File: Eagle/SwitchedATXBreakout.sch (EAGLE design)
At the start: 51 parts, among them K1 ALF1P05, K2 ALF1P05, K3 ALF1P05, K4 ALF1P05, K5 ALF1P05, X1 22-23-2091, X2 5566-24

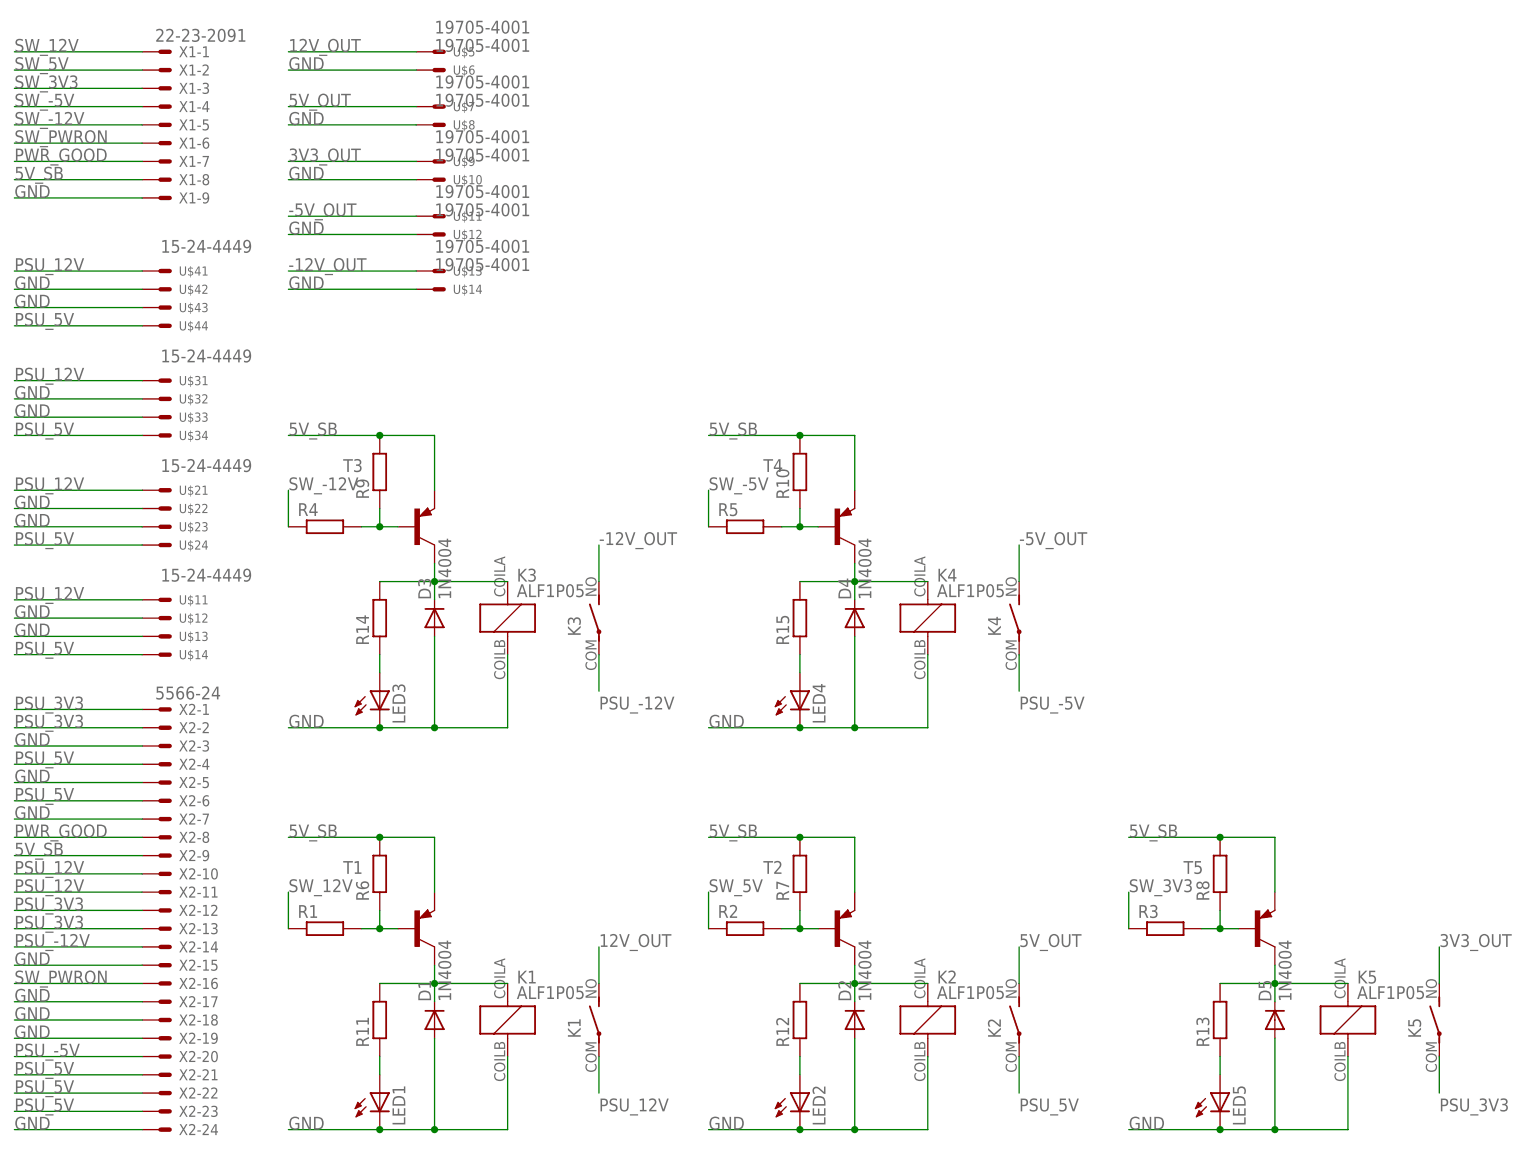
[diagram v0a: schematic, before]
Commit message: Start board layout
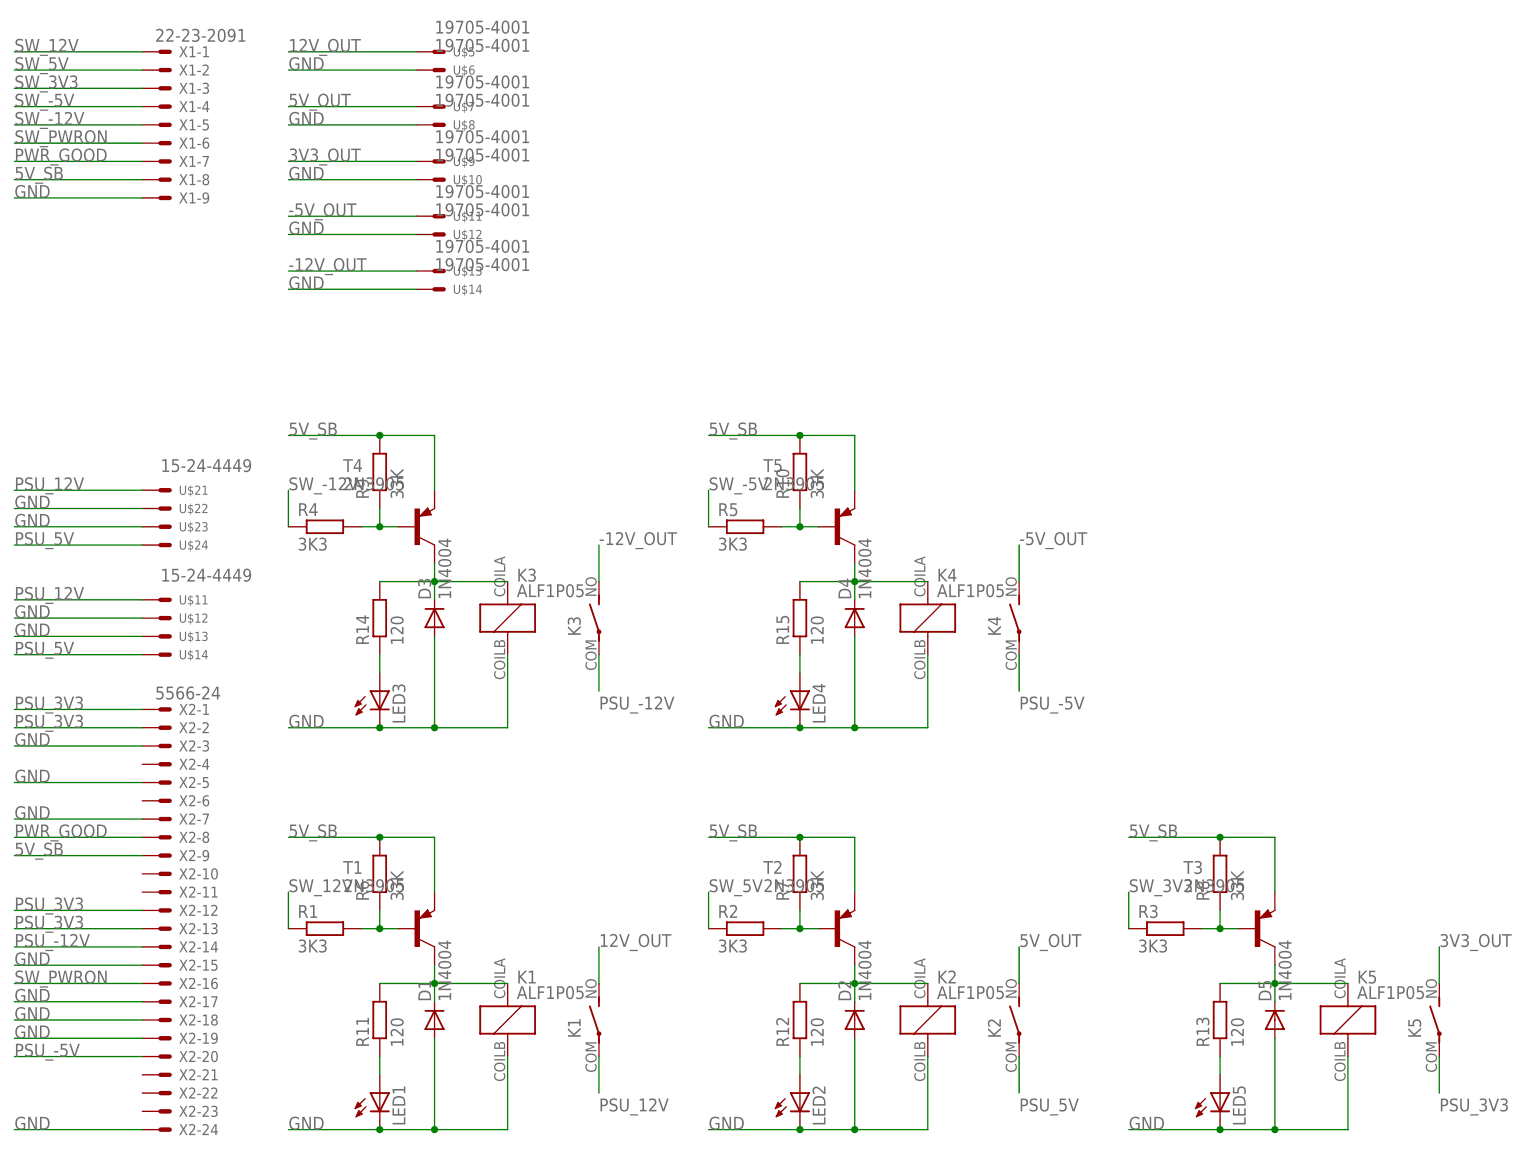
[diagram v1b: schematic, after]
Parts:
- removed U$3, U$4: 15-24-4449, con-molex-additional:15-24-4449
- LED1, LED2, LED3, LED4, LED5: device led:LED5MM -> led:LED3MM
- R1, R2, R3, R4, R5: value (none) -> 3K3; device resistor:R-EU_0204/5 -> resistor:R-EU_0204/7
- R10, R6, R7, R8, R9: value (none) -> 33K; device resistor:R-EU_0204/5 -> resistor:R-EU_0204/7
- R11, R12, R13, R14, R15: value (none) -> 120; device resistor:R-EU_0204/5 -> resistor:R-EU_0204/7
- T1, T2, T3, T4, T5: value (none) -> 2N3905; device transistor:-PNP-TO92 -> transistor:BC636-PNP-TO92-BCE
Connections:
- net GND: no longer U$32.P$1, U$33.P$1, U$42.P$1, U$43.P$1
- net N$11: now also T5.C; no longer T4.C
- net N$14: now also T3.C; no longer T5.C
- net N$2: now also T4.B; no longer T3.B
- net N$5: now also T5.B; no longer T4.B
- net N$7: now also T3.B; no longer T5.B
- net N$8: now also T4.C; no longer T3.C
- net PSU_12V: no longer U$31.P$1, U$41.P$1, X2-10.S, X2-11.S
- net PSU_5V: no longer U$34.P$1, U$44.P$1, X2-21.S, X2-22.S, X2-23.S, X2-4.S, X2-6.S
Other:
- moved on the sheet: T3, T4, T5

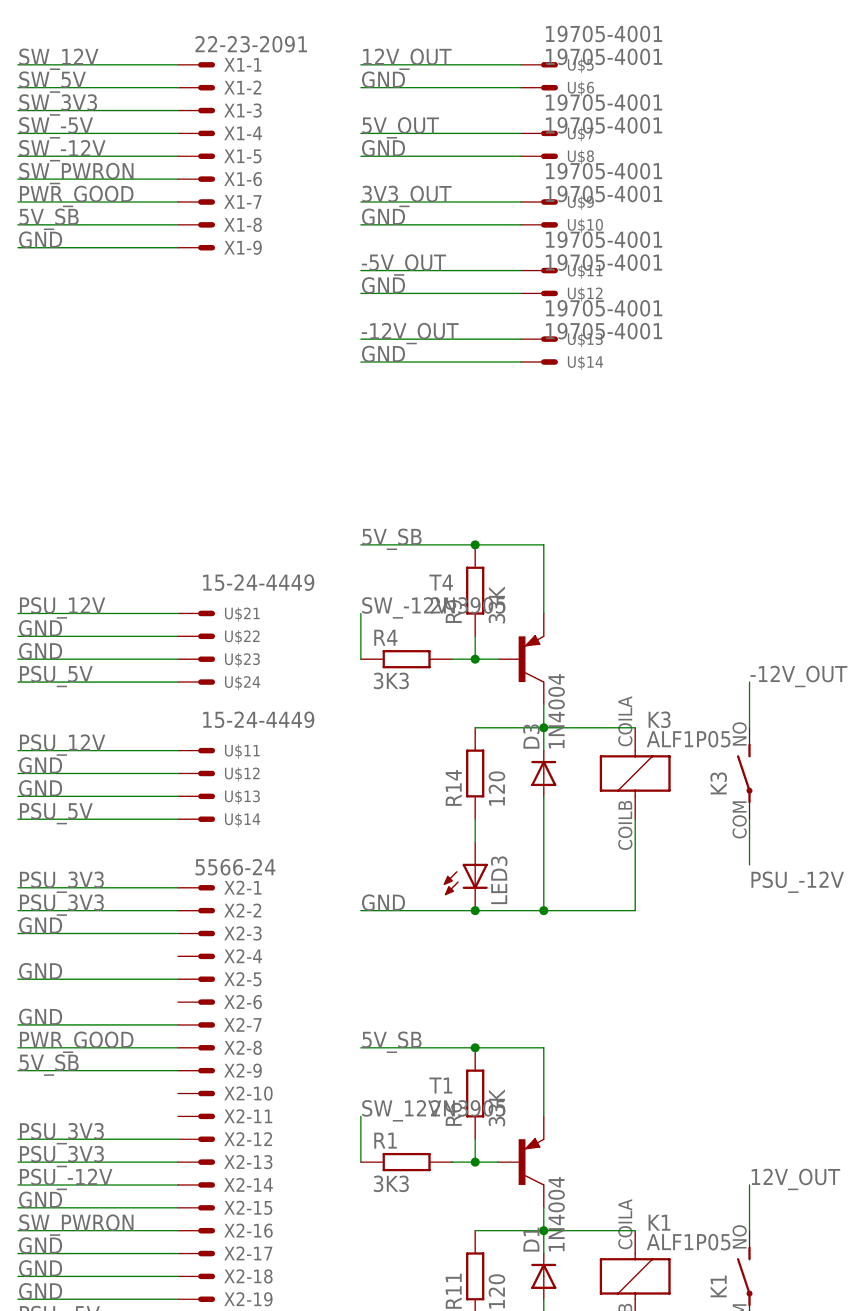
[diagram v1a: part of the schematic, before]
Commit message: Finish board layout
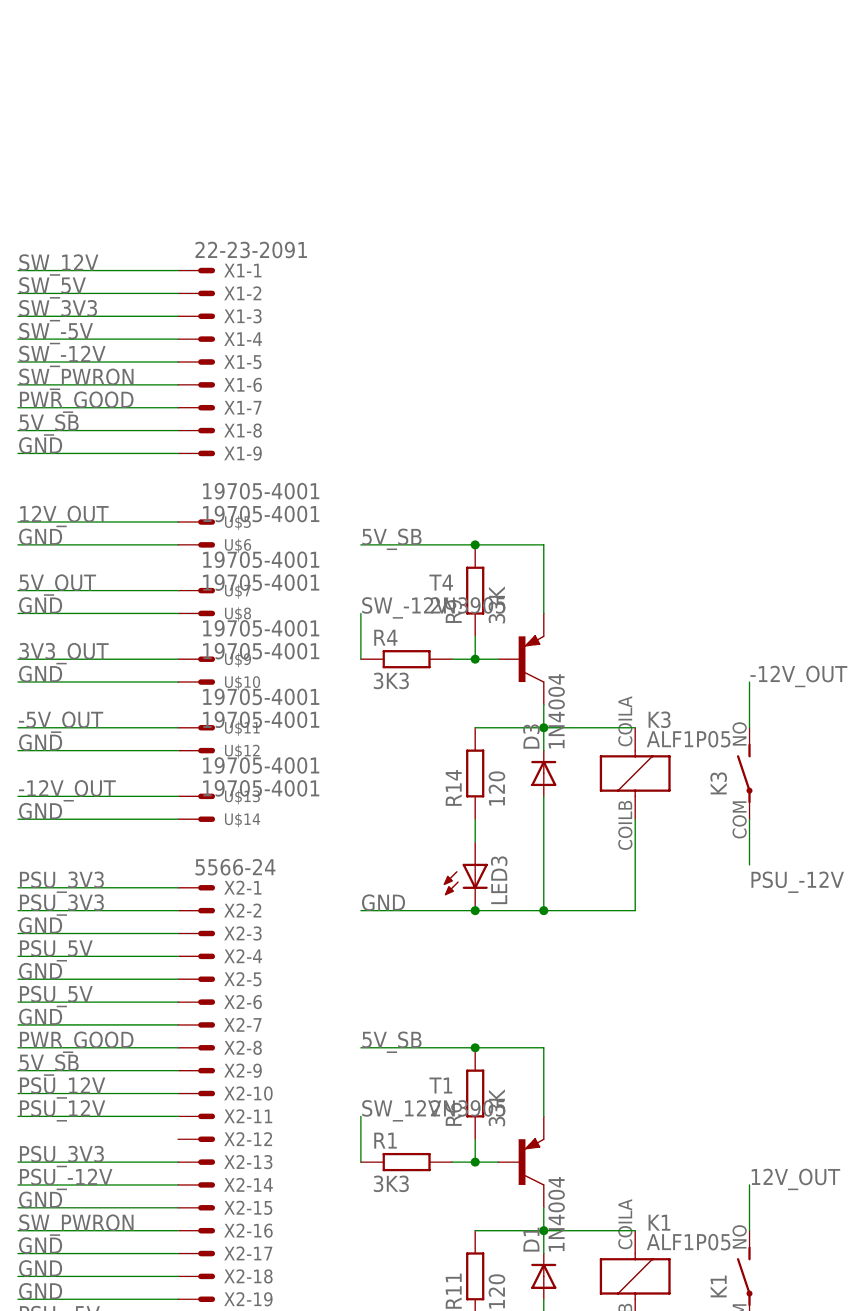
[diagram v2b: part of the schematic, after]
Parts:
- removed U$1, U$2: 15-24-4449, con-molex-additional:15-24-4449
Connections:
- net GND: no longer U$12.P$1, U$13.P$1, U$22.P$1, U$23.P$1
- net PSU_12V: now also X2-10.S, X2-11.S; no longer U$11.P$1, U$21.P$1
- net PSU_3V3: no longer X2-12.S
- net PSU_5V: now also X2-4.S, X2-6.S; no longer U$14.P$1, U$24.P$1
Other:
- moved on the sheet: U$10, U$11, U$12, U$13, U$14, U$5, U$6, U$7, U$8, U$9, X1-1, X1-2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

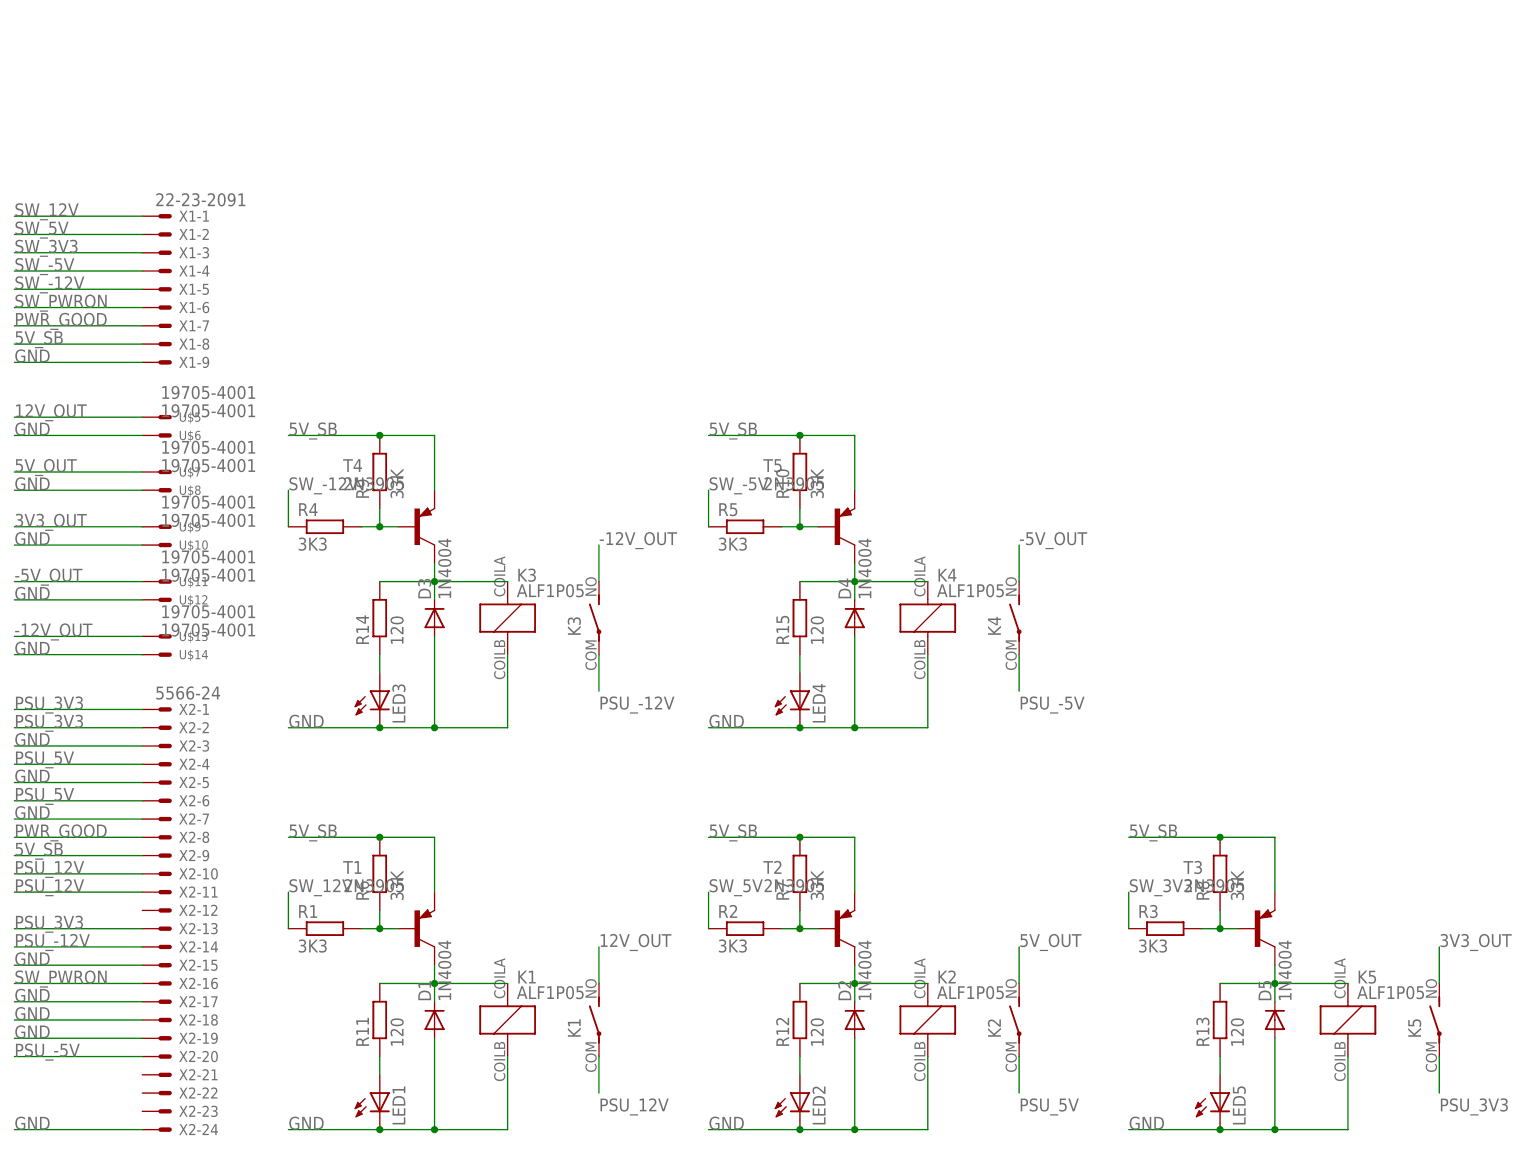
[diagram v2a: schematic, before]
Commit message: Updated board layout
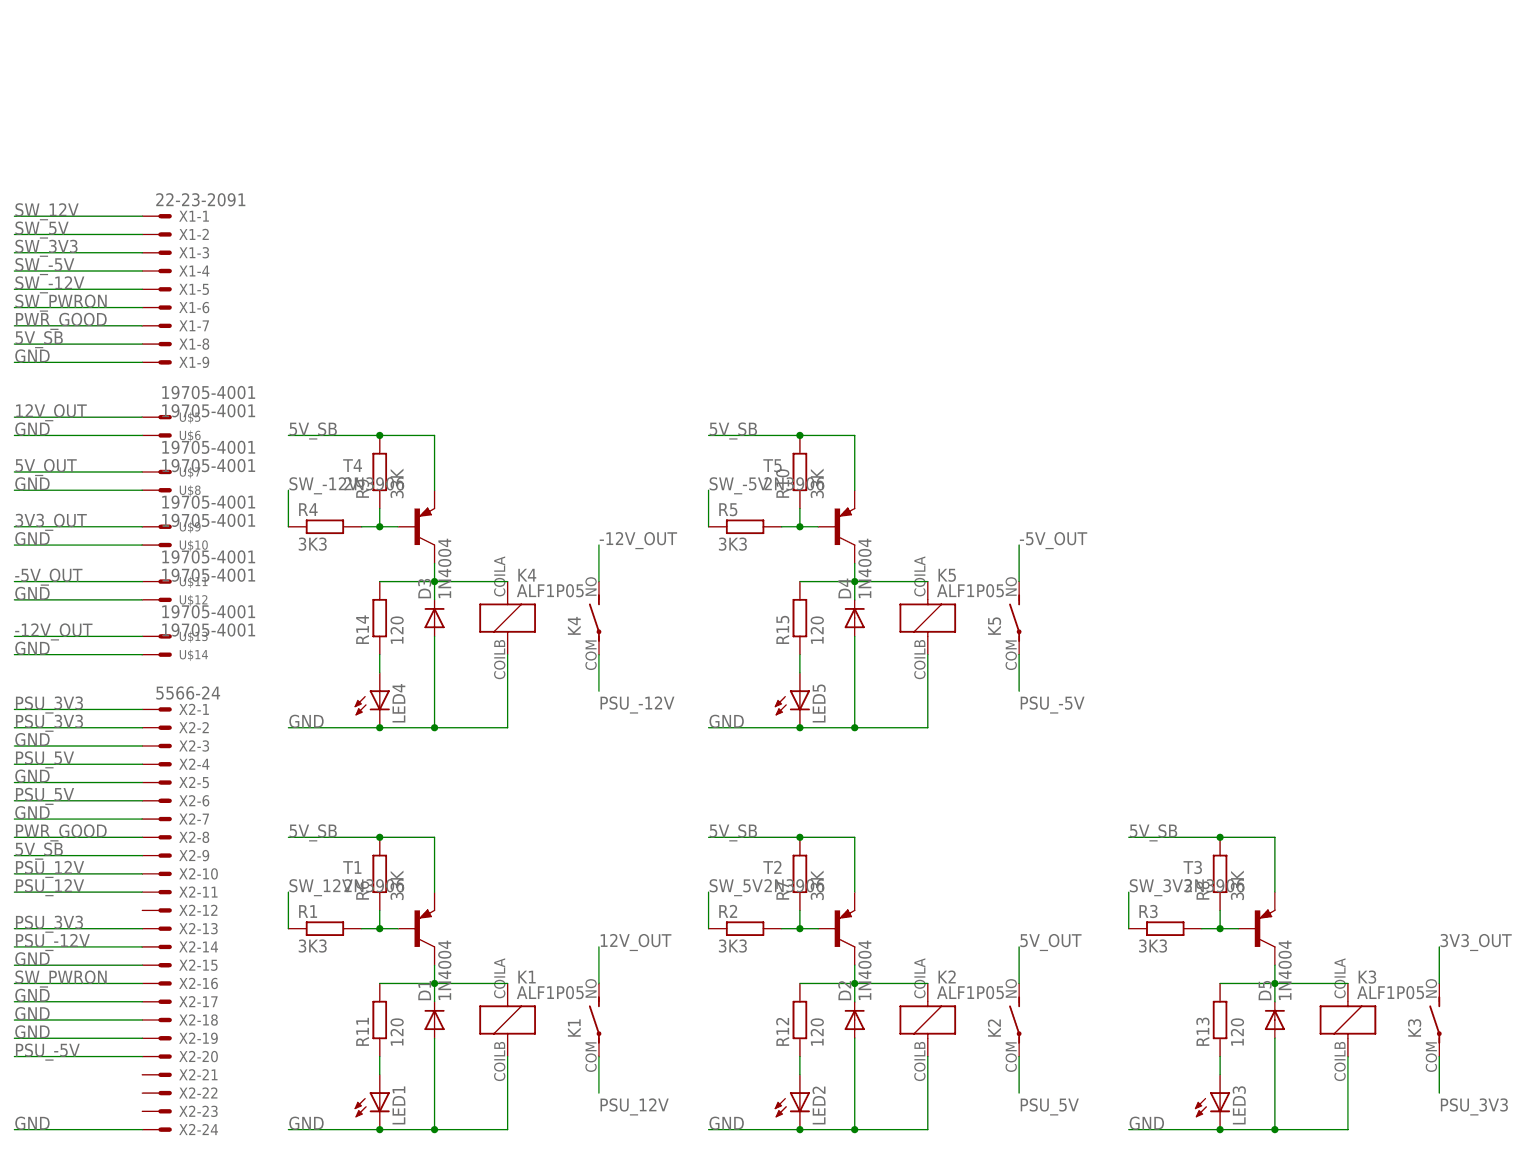
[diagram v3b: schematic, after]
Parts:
- T1, T2, T3, T4, T5: value 2N3905 -> 2N3906; device transistor:BC636-PNP-TO92-BCE -> transistor-neu-to92:-PNP-TO92-EBC
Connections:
- net -12V_OUT: now also K41.S; no longer K31.S
- net -5V_OUT: now also K51.S; no longer K41.S
- net 3V3_OUT: now also K31.S; no longer K51.S
- net N$11: now also K5_.1; no longer K4_.1
- net N$12: now also LED3.A; no longer LED5.A
- net N$13: now also LED5.A; no longer LED4.A
- net N$14: now also K3_.1; no longer K5_.1
- net N$15: now also LED4.A; no longer LED3.A
- net N$8: now also K4_.1; no longer K3_.1
- net PSU_-12V: now also K41.P; no longer K31.P
- net PSU_-5V: now also K51.P; no longer K41.P
- net PSU_3V3: now also K31.P; no longer K51.P
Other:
- moved on the sheet: K3, K4, K5, LED3, LED4, LED5
